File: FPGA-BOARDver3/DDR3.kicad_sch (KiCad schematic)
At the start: 24 parts, among them IC1 IS43TR16256B-125KBLI

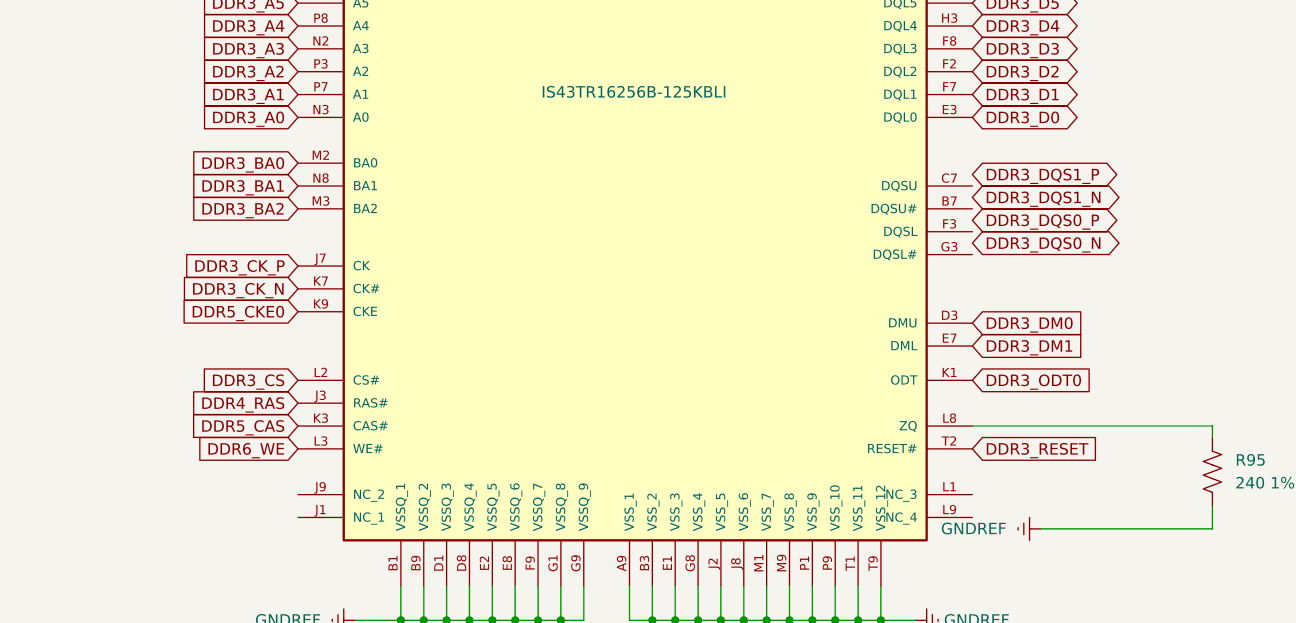
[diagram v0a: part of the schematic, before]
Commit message: updated schematic and layout
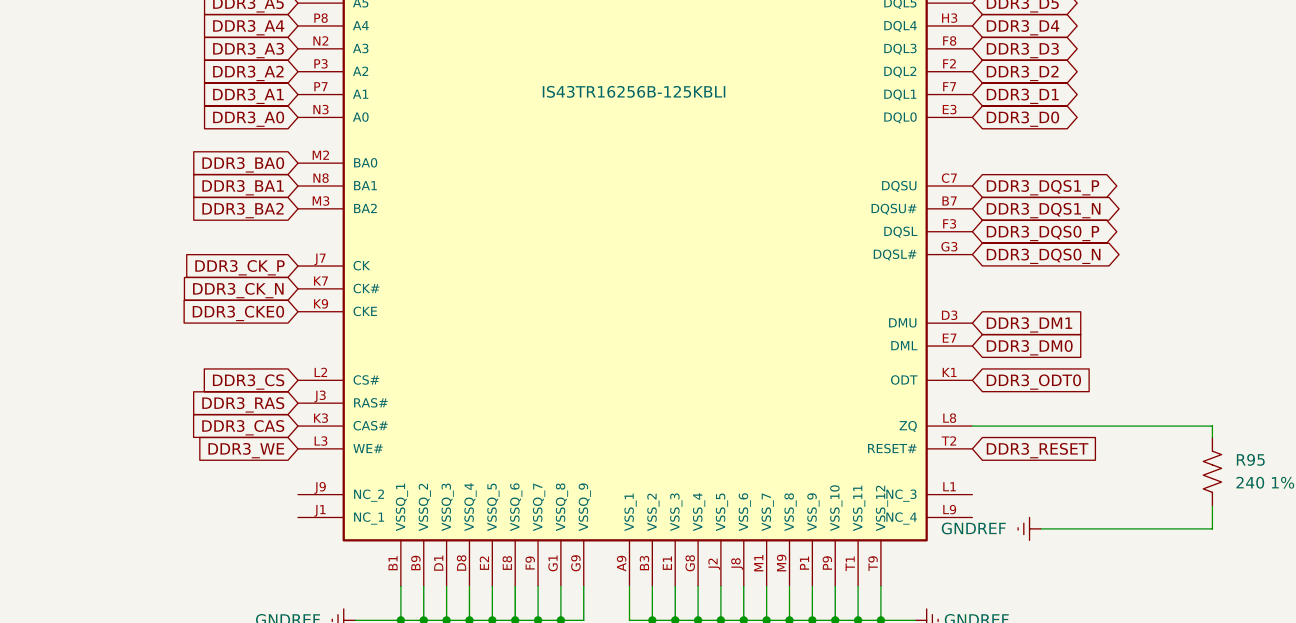
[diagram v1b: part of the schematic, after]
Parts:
- C34, C35: LCSC PN (none) -> c15195
- C36, C37, C38, C39, C40, C41, C42, C43, C44, C45, C46, C47, C48, C49, C50, C51: LCSC PN (none) -> c307434
- C82, C83: LCSC PN (none) -> c92361
- C84: LCSC PN (none) -> c84705
- IC1: LCSC PN (none) -> C1349408
- R95: LCSC PN (none) -> C114755
- R96: LCSC PN (none) -> C105871
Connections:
- net DDR3_DM0: now also IC1.E7 (DML); no longer IC1.D3 (DMU)
- net DDR3_DM1: now also IC1.D3 (DMU); no longer IC1.E7 (DML)
- net DDR3_DQS0_N: now also IC1.G3 (DQSL#)
- net DDR3_DQS0_P: now also IC1.F3 (DQSL)
- net DDR3_DQS1_N: now also IC1.B7 (DQSU#)
- net DDR3_DQS1_P: now also IC1.C7 (DQSU)
- net DDR4_RAS renamed DDR3_RAS
- net DDR5_CAS renamed DDR3_CAS
- net DDR5_CKE0 renamed DDR3_CKE0
- net DDR6_WE renamed DDR3_WE
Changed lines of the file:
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@@
 		)
 	)
-	(global_label "DDR3_DM0"
+	(global_label "DDR3_DM1"
 		(shape input)
 		(at 121.92 113.03 0)
@@
 		)
 	)
-	(global_label "DDR6_WE"
+	(global_label "DDR3_WE"
 		(shape input)
 		(at 46.99 127 180)
@@
 	(global_label "DDR3_DQS1_P"
 		(shape bidirectional)
-		(at 121.92 96.52 0)
+		(at 121.92 97.79 0)
 		(fields_autoplaced yes)
 		(effects
@@
 		)
 		(property "Intersheetrefs" "${INTERSHEET_REFS}"
-			(at 139.2607 96.52 0)
+			(at 139.2607 97.79 0)
 			(effects
 				(font
@@
 	(global_label "DDR3_DQS0_N"
 		(shape bidirectional)
-		(at 121.92 104.14 0)
+		(at 121.92 105.41 0)
 		(fields_autoplaced yes)
 		(effects
@@
 		)
 		(property "Intersheetrefs" "${INTERSHEET_REFS}"
-			(at 139.3212 104.14 0)
+			(at 139.3212 105.41 0)
 			(effects
 				(font
@@
 	(global_label "DDR3_DQS0_P"
 		(shape bidirectional)
-		(at 121.92 101.6 0)
+		(at 121.92 102.87 0)
 		(fields_autoplaced yes)
 		(effects
@@
 		)
 		(property "Intersheetrefs" "${INTERSHEET_REFS}"
-			(at 139.2607 101.6 0)
+			(at 139.2607 102.87 0)
 			(effects
 				(font
@@
 	(global_label "DDR3_DQS1_N"
 		(shape bidirectional)
-		(at 121.92 99.06 0)
+		(at 121.92 100.33 0)
 		(fields_autoplaced yes)
 		(effects
@@
 		)
 		(property "Intersheetrefs" "${INTERSHEET_REFS}"
-			(at 139.3212 99.06 0)
+			(at 139.3212 100.33 0)
 			(effects
 				(font
@@
 		)
 	)
-	(global_label "DDR5_CKE0"
+	(global_label "DDR3_CKE0"
 		(shape input)
 		(at 46.99 111.76 180)
@@
 		)
 	)
-	(global_label "DDR3_DM1"
+	(global_label "DDR3_DM0"
 		(shape input)
 		(at 121.92 115.57 0)
@@
 		)
 	)
-	(global_label "DDR4_RAS"
+	(global_label "DDR3_RAS"
 		(shape input)
 		(at 46.99 121.92 180)
@@
 		)
 	)
-	(global_label "DDR5_CAS"
+	(global_label "DDR3_CAS"
 		(shape input)
 		(at 46.99 124.46 180)
@@
 			)
 		)
-		(property "lcsc#" ""
+		(property "LCSC PN" "c307434"
 			(at 203.2 62.23 0)
 			(effects
@@
 			)
 		)
-		(property "lcsc#" ""
+		(property "LCSC PN" "c307434"
 			(at 233.68 81.28 0)
 			(effects
@@
 			)
 		)
-		(property "lcsc#" ""
+		(property "LCSC PN" "c15195"
 			(at 40.64 34.29 0)
 			(effects
@@
 			)
 		)
-		(property "lcsc#" ""
+		(property "LCSC PN" "c307434"
 			(at 182.88 62.23 0)
 			(effects
@@
 			)
 		)
-		(property "lcsc#" ""
+		(property "LCSC PN" "c307434"
 			(at 243.84 81.28 0)
 			(effects
@@
 			)
 		)
-		(property "lcsc#" ""
+		(property "LCSC PN" "c92361"
 			(at 182.88 100.33 0)
 			(effects
@@
 			)
 		)
-		(property "lcsc#" ""
+		(property "LCSC PN" "c307434"
 			(at 254 81.28 0)
 			(effects
@@
 			)
 		)
-		(property "lcsc#" ""
+		(property "LCSC PN" "c307434"
 			(at 213.36 81.28 0)
 			(effects
@@
 			)
 		)
-		(property "lcsc#" ""
+		(property "LCSC PN" "c307434"
 			(at 213.36 62.23 0)
 			(effects
@@
 			)
 		)
-		(property "lcsc#" ""
+		(property "LCSC PN" "c307434"
 			(at 193.04 62.23 0)
 			(effects
@@
 			)
 		)
-		(property "lcsc#" ""
+		(property "LCSC PN" "c307434"
 			(at 182.88 81.28 0)
 			(effects
@@
 			)
 		)
-		(property "lcsc#" ""
+		(property "LCSC PN" "c15195"
 			(at 30.48 43.18 0)
 			(effects
@@
 			)
 		)
-		(property "lcsc#" ""
+		(property "LCSC PN" "C114755"
 			(at 148.59 129.54 0)
 			(effects
@@
 			)
 		)
-		(property "lcsc#" ""
+		(property "LCSC PN" "c307434"
 			(at 223.52 81.28 0)
 			(effects
@@
 			)
 		)
-		(property "lcsc#" ""
+		(property "LCSC PN" "c307434"
 			(at 193.04 81.28 0)
 			(effects
@@
 			)
 		)
-		(property "lcsc#" ""
+		(property "LCSC PN" "c307434"
 			(at 254 62.23 0)
 			(effects
@@
 			)
 		)
-		(property "lcsc#" ""
+		(property "LCSC PN" "C1349408"
 			(at 86.36 15.24 0)
 			(effects
@@
 			)
 		)
-		(property "lcsc#" ""
+		(property "LCSC PN" "C105871"
 			(at 199.39 124.46 0)
 			(effects
@@
 			)
 		)
-		(property "lcsc#" ""
+		(property "LCSC PN" "c92361"
 			(at 193.04 100.33 0)
 			(effects
@@
 			)
 		)
-		(property "lcsc#" ""
+		(property "LCSC PN" "c307434"
 			(at 223.52 62.23 0)
 			(effects
@@
 			)
 		)
-		(property "lcsc#" ""
+		(property "LCSC PN" "c307434"
 			(at 243.84 62.23 0)
 			(effects
@@
 			)
 		)
-		(property "lcsc#" ""
+		(property "LCSC PN" "c307434"
 			(at 233.68 62.23 0)
 			(effects
@@
 			)
 		)
-		(property "lcsc#" ""
+		(property "LCSC PN" "c84705"
 			(at 203.2 100.33 0)
 			(effects
@@
 			)
 		)
-		(property "lcsc#" ""
+		(property "LCSC PN" "c307434"
 			(at 203.2 81.28 0)
 			(effects
